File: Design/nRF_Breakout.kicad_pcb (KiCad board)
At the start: 2 copper layers, 26 x 59 mm, 17 parts, among them IC1 LM1117, P1 CONN_01X18, P10 CONN_01X01, P2 CONN_01X08, P3 CONN_01X18, P4 CONN_01X02, P5 CONN_01X08, P7 CONN_01X01, P8 CONN_01X01, P9 CONN_01X01, U1 nRF51822

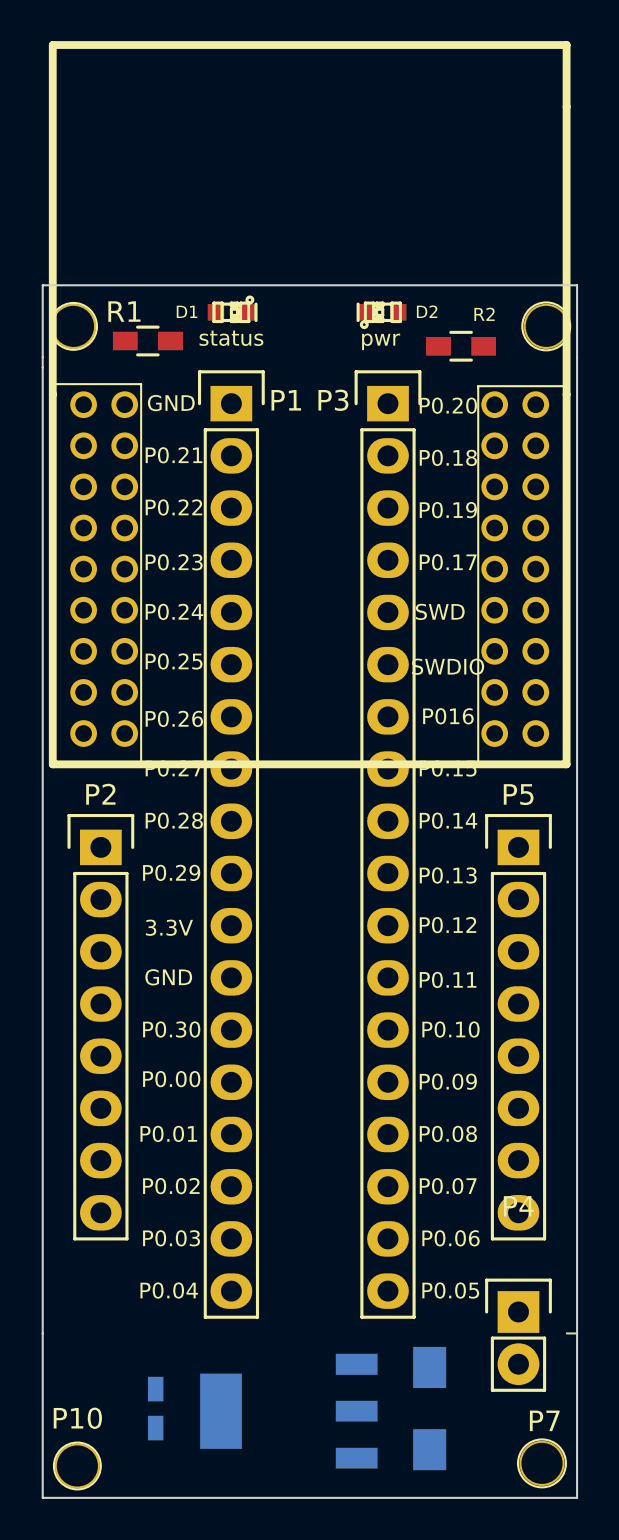
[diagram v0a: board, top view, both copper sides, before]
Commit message: Corrected File
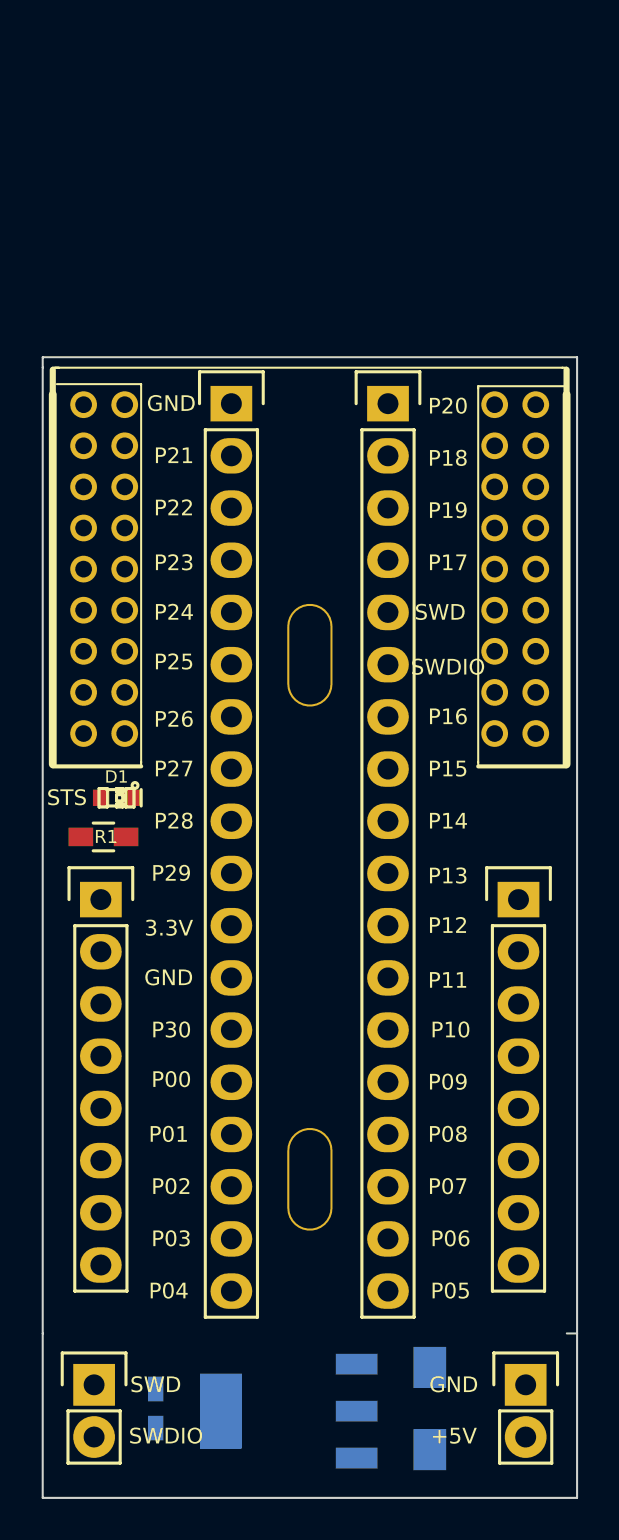
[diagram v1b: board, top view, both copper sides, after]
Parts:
- removed D2: LED, ee:LED-0603_NEW
- removed P10, P9: CONN_01X01, Connect:1pin
- removed R2: 470r, Resistors_SMD:R_0603_HandSoldering
- added P6: CONN_01X02, Pin_Headers:Pin_Header_Straight_1x02, F.Cu at (163.5, 96.0)
- moved D1 24.3 mm to (164.6, 67.4)
- moved R1 24.2 mm to (164.0, 69.3), turned to 180 degrees
- moved P8 19.7 mm to (174.0, 60.5)
- moved P7 17.8 mm to (174.0, 86.0)
- moved P4 3.56 mm to (184.5, 96.0)
- moved P2 2.54 mm to (163.8, 72.4)
- moved P5 2.54 mm to (184.2, 72.4)
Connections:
- net +3.3VP renamed Net-(C2-Pad1)
- net ST_LED renamed Net-(P1-Pad2)
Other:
- board size 26 x 59 mm -> 26 x 55.5 mm
- board text added: "+5V"
- board text added: "P00"
- board text added: "P01"
- board text added: "P02"
- board text added: "P03"
- board text added: "P04"
- board text added: "P05"
- board text added: "P06"
- board text added: "P07"
- board text added: "P08"
- board text added: "P09"
- board text added: "P10"
- board text added: "P11"
- board text added: "P12"
- board text added: "P13"
- board text added: "P14"
- board text added: "P15"
- board text added: "P16"
- board text added: "P17"
- board text added: "P18"
- board text added: "P19"
- board text added: "P20"
- board text added: "P21"
- board text added: "P22"
- board text added: "P23"
- board text added: "P24"
- board text added: "P25"
- board text added: "P26"
- board text added: "P27"
- board text added: "P28"
- board text added: "P29"
- board text added: "P30"
- board text added: "STS"
- board text removed: "P0.00"
- board text removed: "P0.01"
- board text removed: "P0.02"
- board text removed: "P0.03"
- board text removed: "P0.04"
- board text removed: "P0.05"
- board text removed: "P0.06"
- board text removed: "P0.07"
- board text removed: "P0.08"
- board text removed: "P0.09"
- board text removed: "P0.10"
- board text removed: "P0.11"
- board text removed: "P0.12"
- board text removed: "P0.13"
- board text removed: "P0.14"
- board text removed: "P0.15"
- board text removed: "P0.17"
- board text removed: "P0.18"
- board text removed: "P0.19"
- board text removed: "P0.20"
- board text removed: "P0.21"
- board text removed: "P0.22"
- board text removed: "P0.23"
- board text removed: "P0.24"
- board text removed: "P0.25"
- board text removed: "P0.26"
- board text removed: "P0.27"
- board text removed: "P0.28"
- board text removed: "P0.29"
- board text removed: "P0.30"
- board text removed: "P016"
- board text removed: "pwr"
- board text removed: "status"
